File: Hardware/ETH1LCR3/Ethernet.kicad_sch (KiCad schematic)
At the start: 25 parts, among them J201 RJ45_Wuerth_7499010121A, U201 LAN8742A, Y201 NX5032GA-25

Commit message: Schematic
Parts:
- Y201: footprint ETH1HMSR-SMS:NX5032GA -> (none)
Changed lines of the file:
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@@
 			)
 		)
-		(property "Footprint" "ETH1HMSR-SMS:NX5032GA"
+		(property "Footprint" ""
 			(at 80.01 125.73 0)
 			(effects

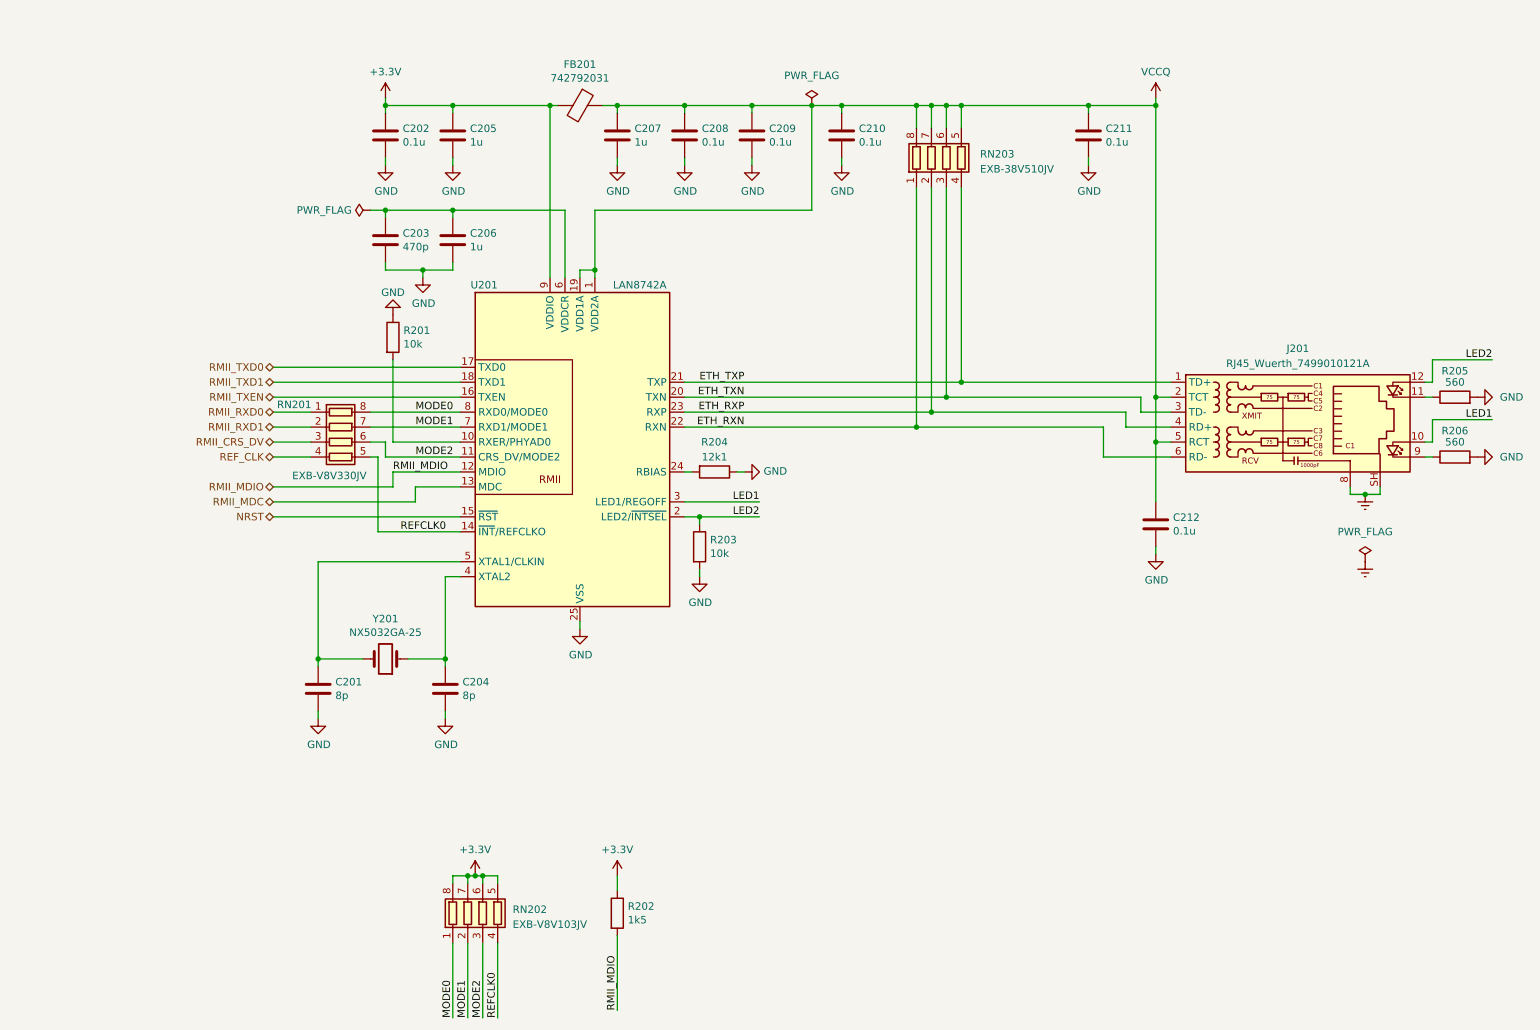
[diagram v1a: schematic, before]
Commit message: Hardware
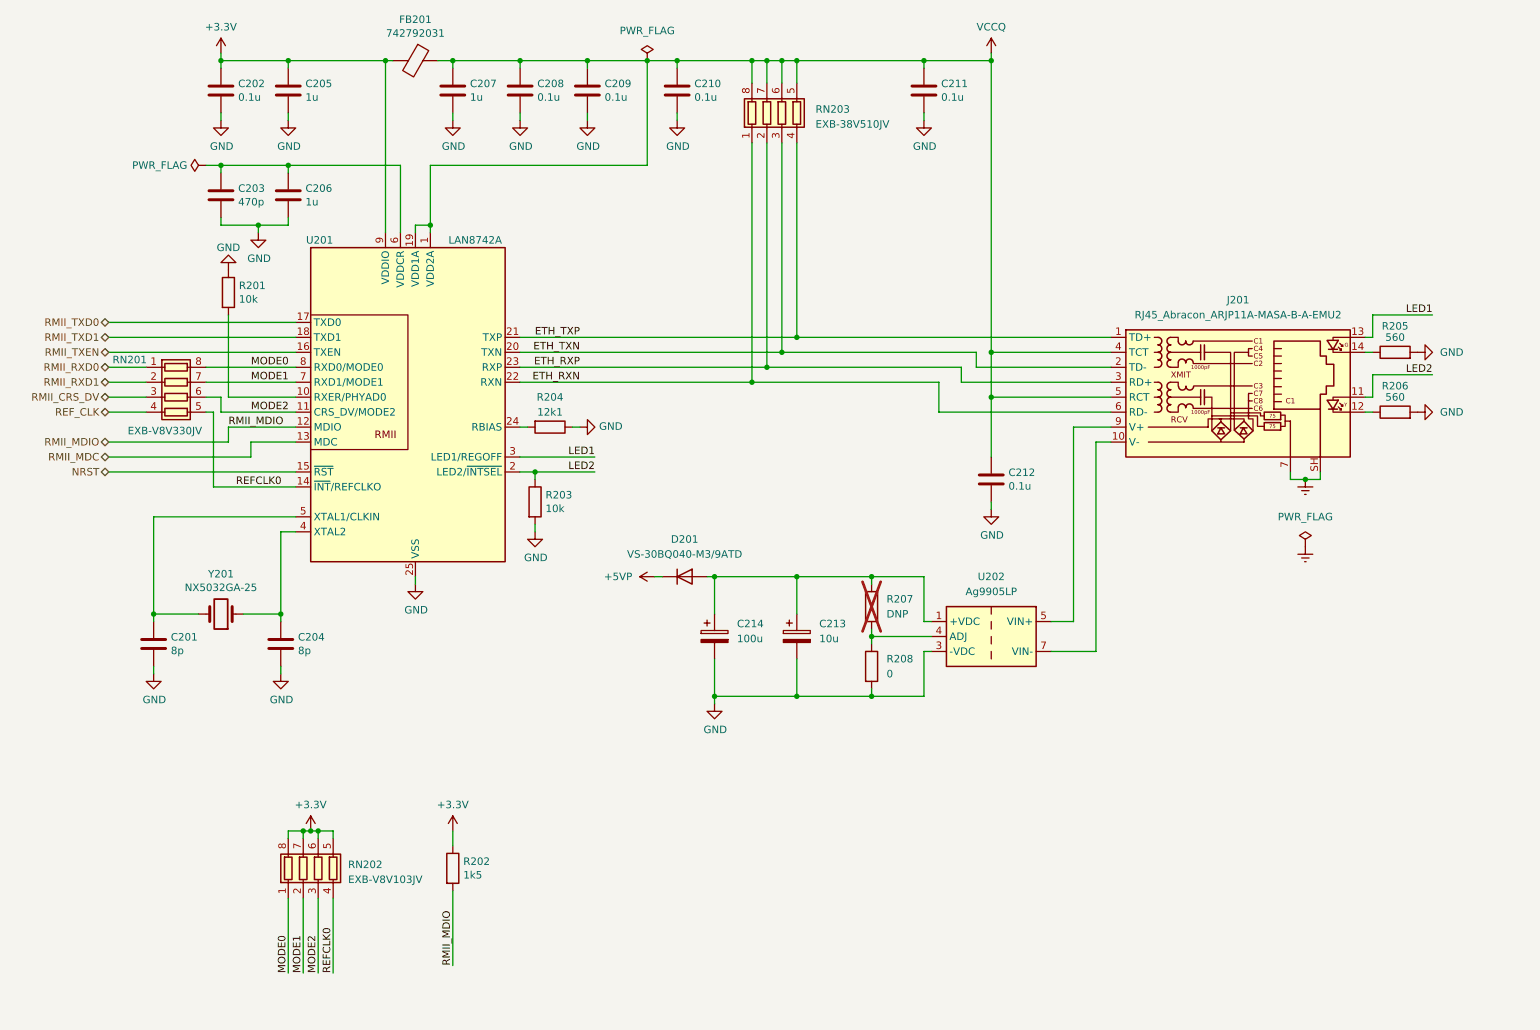
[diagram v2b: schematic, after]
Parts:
- removed J201: RJ45_Wuerth_7499010121A, Connector_RJ:RJ45_Wuerth_7499010121A_Horizontal, symbol Connector:RJ45_Wuerth_7499010121A
- added C213: 10u, symbol Device:C_Polarized
- added C214: 100u, symbol Device:C_Polarized
- added D201: VS-30BQ040-M3/9ATD, symbol Device:D
- added J201: RJ45_Abracon_ARJP11A-MASA-B-A-EMU2, Connector_RJ:RJ45_Abracon_ARJP11A-MA_Horizontal, symbol Connector:RJ45_Abracon_ARJP11A-MASA-B-A-EMU2
- added R207: DNP, symbol Device:R
- added R208: 0, symbol Device:R
- added U202: Ag9905LP, Converter_DCDC:Converter_DCDC_Silvertel_Ag99xxLP_THT, symbol Converter_DCDC:Ag9905LP
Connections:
- net ETH_RXN: now also J201.6 (RD-)
- net ETH_RXP: now also J201.3 (RD+)
- net ETH_TXN: now also J201.2 (TD-)
- net ETH_TXP: now also J201.1 (TD+)
- net Earth: now also J201.7, J201.SH
- net GND: now also C213.2, C214.2, R208.2, U202.3 (-VDC)
- net LED1: now also J201.13
- net LED2: now also J201.11
- net VCCQ: now also J201.4 (TCT), J201.5 (RCT)
- net at R205.1: now also J201.14
- net at R206.1: now also J201.12
- new net: C213.1, C214.1, D201.2 (A), R207.1, U202.1 (+VDC), U202.2 (+VDC)
- new net: J201.10 (V-), U202.7 (VIN-), U202.8 (VIN-)
- new net: J201.9 (V+), U202.5 (VIN+), U202.6 (VIN+)
- new net: R207.2, R208.1, U202.4 (ADJ)
- new net +5VP: D201.1 (K)
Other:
- moved on the sheet: C201, C202, C203, C204, C205, C206, C207, C208, C209, C210, C211, C212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
